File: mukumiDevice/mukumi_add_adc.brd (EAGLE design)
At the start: 49.2 x 49.6 mm, 151 parts, among them IC1 AD835, IC10 NJM2884, IC11 AD9834, IC12 AD9834, IC13 SIT8002B, IC14 NJM074V, IC2 AD835, IC5 NJM074V, IC6 NJM074V, IC7 NJM074V, IC8 NJM074V, IC9 NJM2884

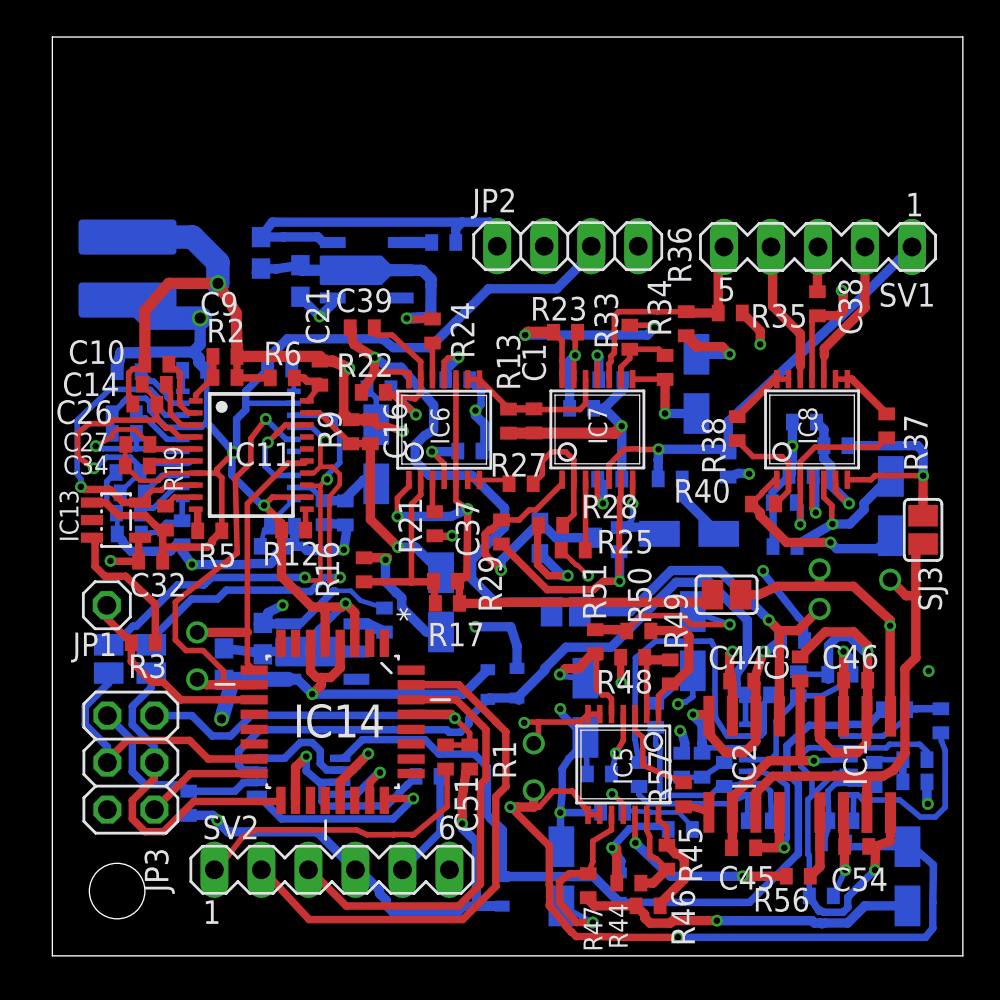
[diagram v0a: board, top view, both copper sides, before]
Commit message: ACカップリングコンデンサをPMLCAPへ変更とadc通信用i2cパスにプルアップ抵抗の追加
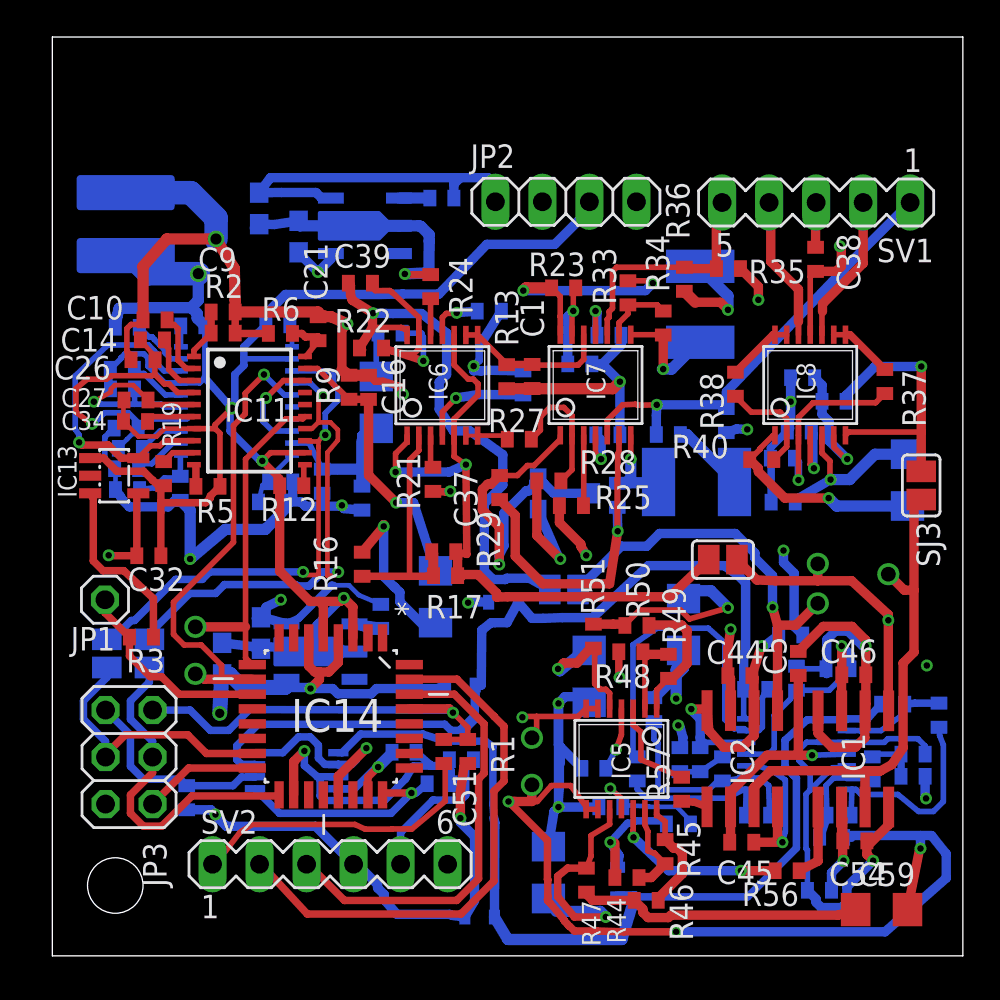
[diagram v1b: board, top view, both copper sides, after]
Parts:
- added R52, R53: 10k, rcl:R0402
- C2: value 0.47u -> (none); device rcl:PANASONIC_B -> rcl:C1206
- C23, C40: device rcl:PANASONIC_B -> rcl:C1812K
- C3, C4, C56, C57, C58, C59: device rcl:PANASONIC_B -> rcl:C1206
- moved C50 4.67 mm to (25.4, 31.0), turned to 90 degrees
- moved D3 4.44 mm to (24.4, 19.1), turned to 90 degrees
- moved C23 4.30 mm to (35.0, 35.2), turned to 90 degrees
- moved C49 4.07 mm to (23.6, 34.8)
- moved R26 3.06 mm to (18.2, 33.6)
- moved C40 2.83 mm to (34.8, 25.6), turned to 180 degrees
- moved C4 2.80 mm to (17.5, 29.9), turned to 90 degrees
- moved C24 2.40 mm to (11.2, 40.4)
- moved C38 2.40 mm to (41.2, 37.6)
- moved JP2 2.40 mm to (27.7, 40.7)
- moved R35 2.40 mm to (36.5, 37.1)
- moved SV1 2.40 mm to (41.3, 40.7)
- moved C1 2.40 mm to (25.9, 31.3)
- moved C10 2.40 mm to (5.55, 34.4)
- moved C12 2.40 mm to (30.1, 33.5)
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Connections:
- net 3.3V_DDS: now also R52.2, R53.1
- net A1: now also C40.1; no longer C40.+
- net AGND: now also C56.2, C58.2; no longer C56.-, C58.-
- net DDS_OUT1: now also C3.1; no longer C3.+
- net DDS_OUT2: now also C4.1; no longer C4.+
- net N$2: now also C56.1; no longer C56.+
- net N$3: now also C58.1; no longer C58.+
- net N$4: now also C57.1; no longer C57.+
- net N$41: now also C23.2; no longer C23.-
- net N$45: now also C4.2; no longer C4.-
- net N$46: now also C40.2; no longer C40.-
- net N$54: now also C2.1; no longer C2.+
- net N$55: now also C2.2; no longer C2.-
- net N$56: now also C23.1; no longer C23.+
- net N$6: now also C59.1; no longer C59.+
- net N$64: now also C3.2; no longer C3.-
- net SCL_AD: now also R52.1
- net SDA_AD: now also R53.2
- net SIG*COS: now also C57.2; no longer C57.-
- net SIG*SIN: now also C59.2; no longer C59.-
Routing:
- net GND: track 206.5 -> 214.8 mm
- net AGND: track 392.9 -> 400.5 mm
- net 3.3V_DDS: track 133.6 -> 140.9 mm
- net AOUT2: track 40.8 -> 47.9 mm
- net AOUT1: track 45.0 -> 50.9 mm
- net +5V: track 128.0 -> 133.7 mm
- net N$48: track 14.5 -> 19.8 mm
- net SIG*SIN: track 43.7 -> 48.7 mm, vias 3 -> 4
- net N$44: track 20.4 -> 25.4 mm
- net -5V: track 111.8 -> 116.3 mm
- net DDS_OUT2: track 5.51 -> 9.89 mm
- net SIN: track 32.8 -> 37.1 mm
- net N$78: track 10.7 -> 14.2 mm
- net N$6: track 19.2 -> 16.1 mm, vias 1 -> 0
- net SIG: track 11.9 -> 14.9 mm
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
